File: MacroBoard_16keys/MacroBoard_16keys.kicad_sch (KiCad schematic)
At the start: 20 parts, among them SW1 SW_DIP_x01, SW10 SW_DIP_x01, SW11 SW_DIP_x01, SW12 SW_DIP_x01, SW13 SW_DIP_x01, SW14 SW_DIP_x01, SW15 SW_DIP_x01, SW16 SW_DIP_x01, SW2 SW_DIP_x01, SW3 SW_DIP_x01, SW4 SW_DIP_x01, SW5 SW_DIP_x01, SW6 SW_DIP_x01, SW7 SW_DIP_x01, SW8 SW_DIP_x01, SW9 SW_DIP_x01

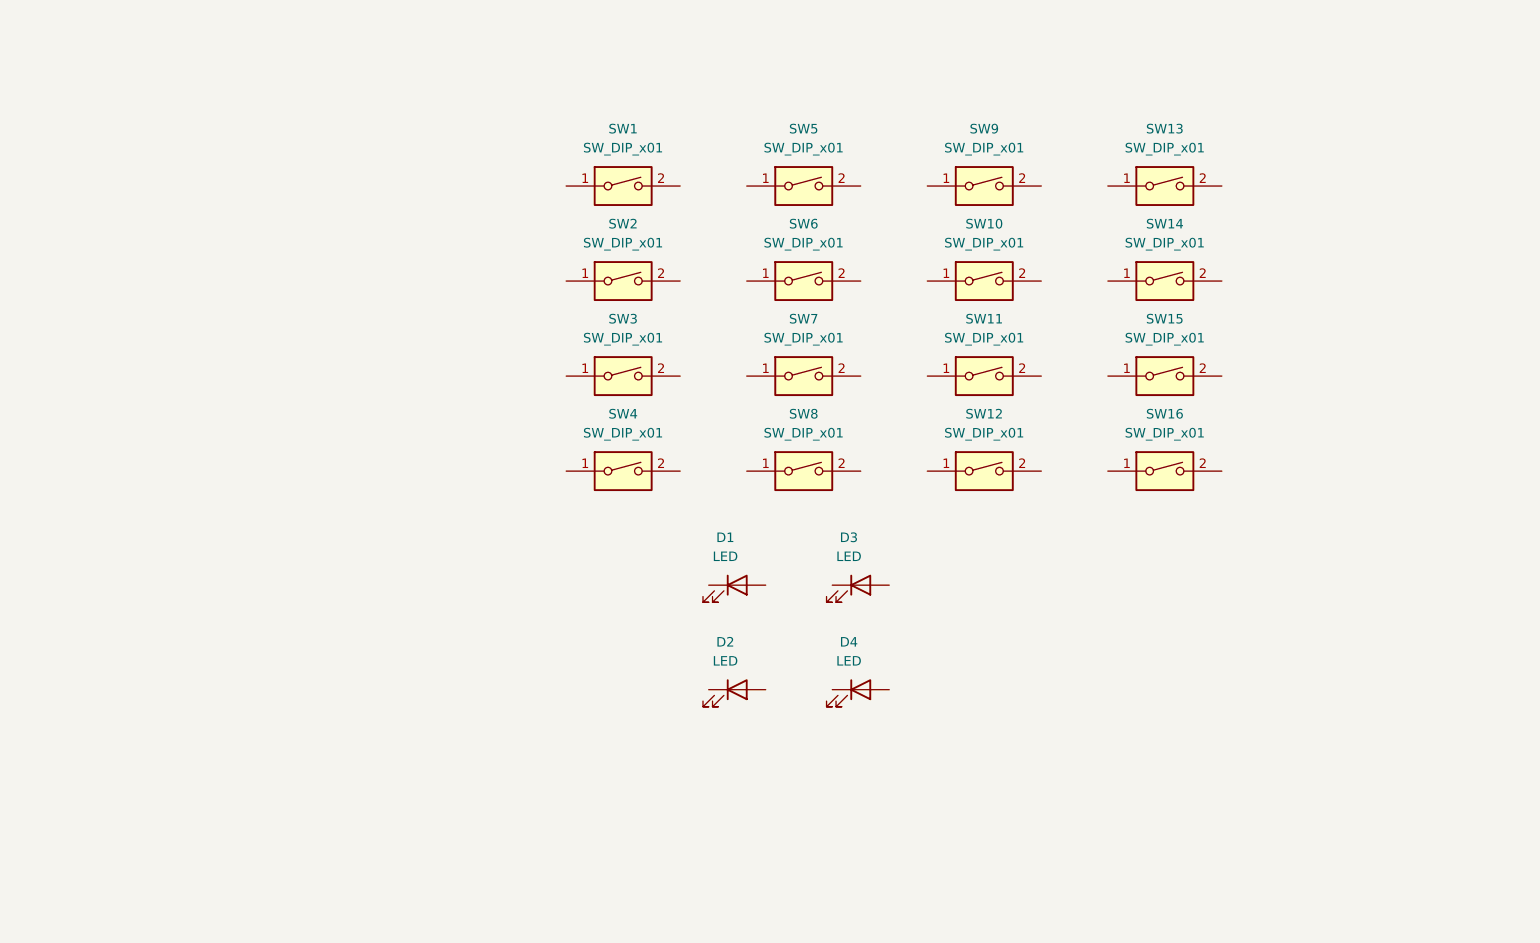
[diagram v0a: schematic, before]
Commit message: Added 3D-model Added Gerber files Added code
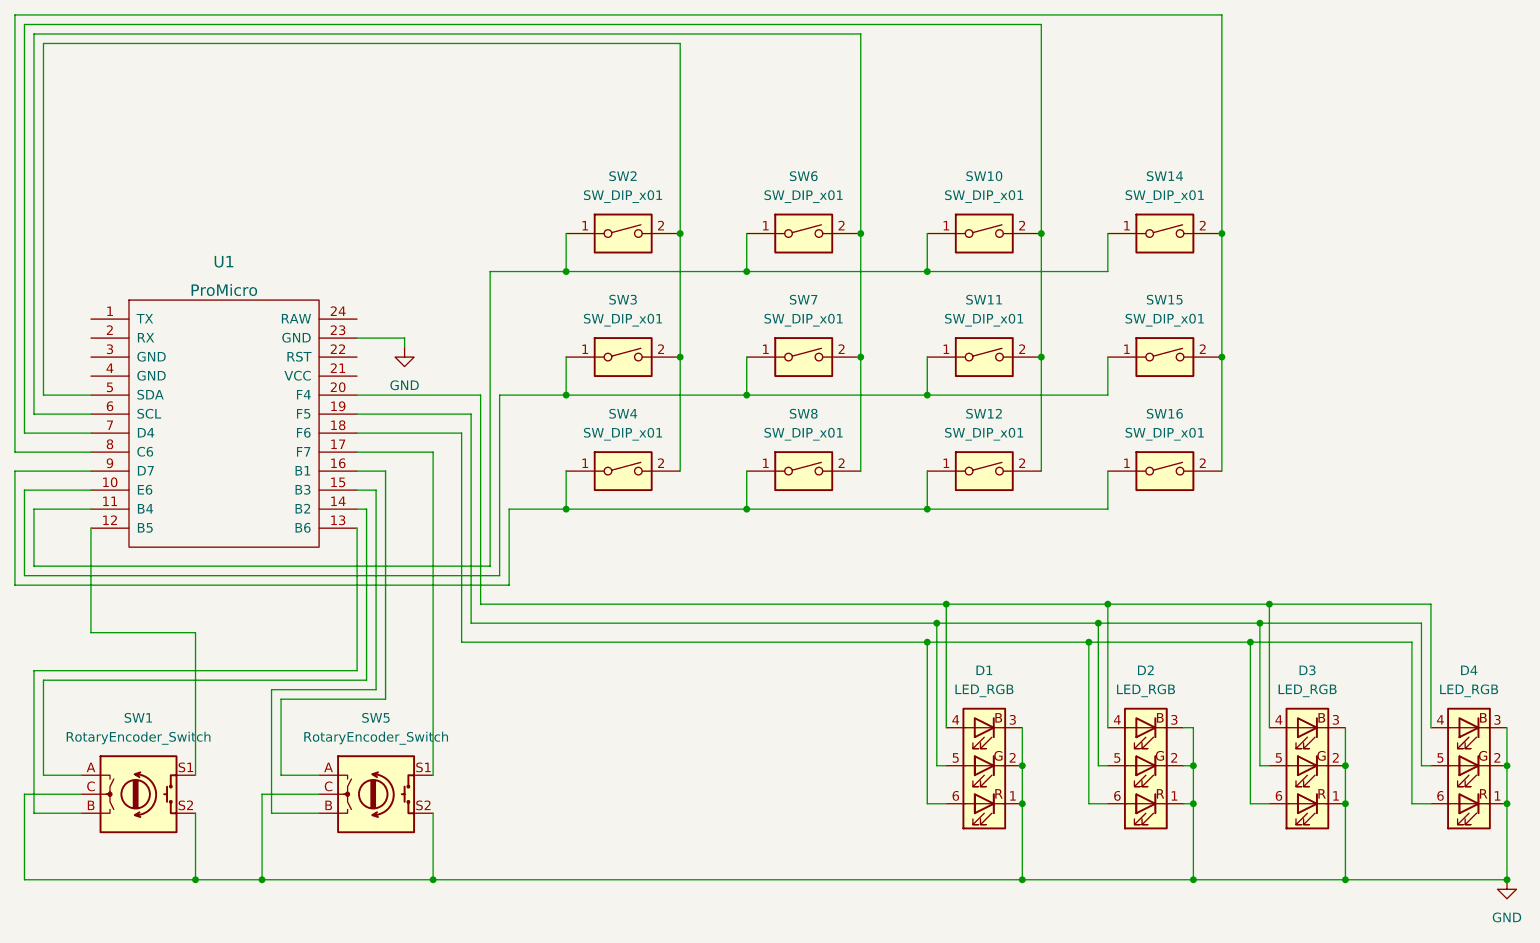
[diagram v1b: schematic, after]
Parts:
- removed D1, D2, D3, D4: LED, LED_SMD:LED_0201_0603Metric_Pad0.64x0.40mm_HandSolder, symbol Device:LED
- removed SW1, SW13, SW5, SW9: SW_DIP_x01, Button_Switch_Keyboard:SW_Cherry_MX_1.00u_PCB, symbol Switch:SW_DIP_x01
- added D1, D2, D3, D4: LED_RGB, LED_SMD:LED_RGB_5050-6, symbol Device:LED_RGB
- added SW1, SW5: RotaryEncoder_Switch, Rotary_Encoder:RotaryEncoder_Alps_EC11E-Switch_Vertical_H20mm, symbol Device:RotaryEncoder_Switch
- added U1: ProMicro, Arduino Micro Pro:ProMicro, symbol Arduino:ProMicro
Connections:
- net at SW16.1: now also SW12.1, SW4.1, SW8.1, U1.9 (D7)
- net at SW16.2: now also SW14.2, SW15.2, U1.8 (C6)
- net at SW15.1: now also SW11.1, SW3.1, SW7.1, U1.10 (E6)
- net at SW11.2: now also SW10.2, SW12.2, U1.7 (D4)
- net at SW7.2: now also SW6.2, SW8.2, U1.6 (SCL)
- net at SW10.1: now also SW14.1, SW2.1, SW6.1, U1.11 (B4)
- net at SW3.2: now also SW2.2, SW4.2, U1.5 (SDA)
- new net: D1.4 (BA), D2.4 (BA), D3.4 (BA), D4.4 (BA), U1.20 (F4)
- new net: D1.5 (GA), D2.5 (GA), D3.5 (GA), D4.5 (GA), U1.19 (F5)
- new net: D1.6 (RA), D2.6 (RA), D3.6 (RA), D4.6 (RA), U1.18 (F6)
- new net: SW1.S1, U1.12 (B5)
- new net: SW1.B, U1.13 (B6)
- new net: SW1.A, U1.14 (B2)
- new net: SW5.B, U1.15 (B3)
- new net: SW5.A, U1.16 (B1)
- new net: SW5.S1, U1.17 (F7)
- new net GND: D1.1 (RK), D1.2 (GK), D1.3 (BK), D2.1 (RK), D2.2 (GK), D2.3 (BK), D3.1 (RK), D3.2 (GK), D3.3 (BK), D4.1 (RK), D4.2 (GK), D4.3 (BK), SW1.C, SW1.S2, SW5.C, SW5.S2, U1.23 (GND)
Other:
- moved on the sheet: SW10, SW11, SW14, SW15, SW2, SW3, SW6, SW7
